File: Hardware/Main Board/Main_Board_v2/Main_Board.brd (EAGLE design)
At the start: 138.4 x 103.8 mm, 54 parts, among them IC1 MBED_MICROCONTROLLER, IC2 NE555, Q1 IRF3704, Q2 BS170

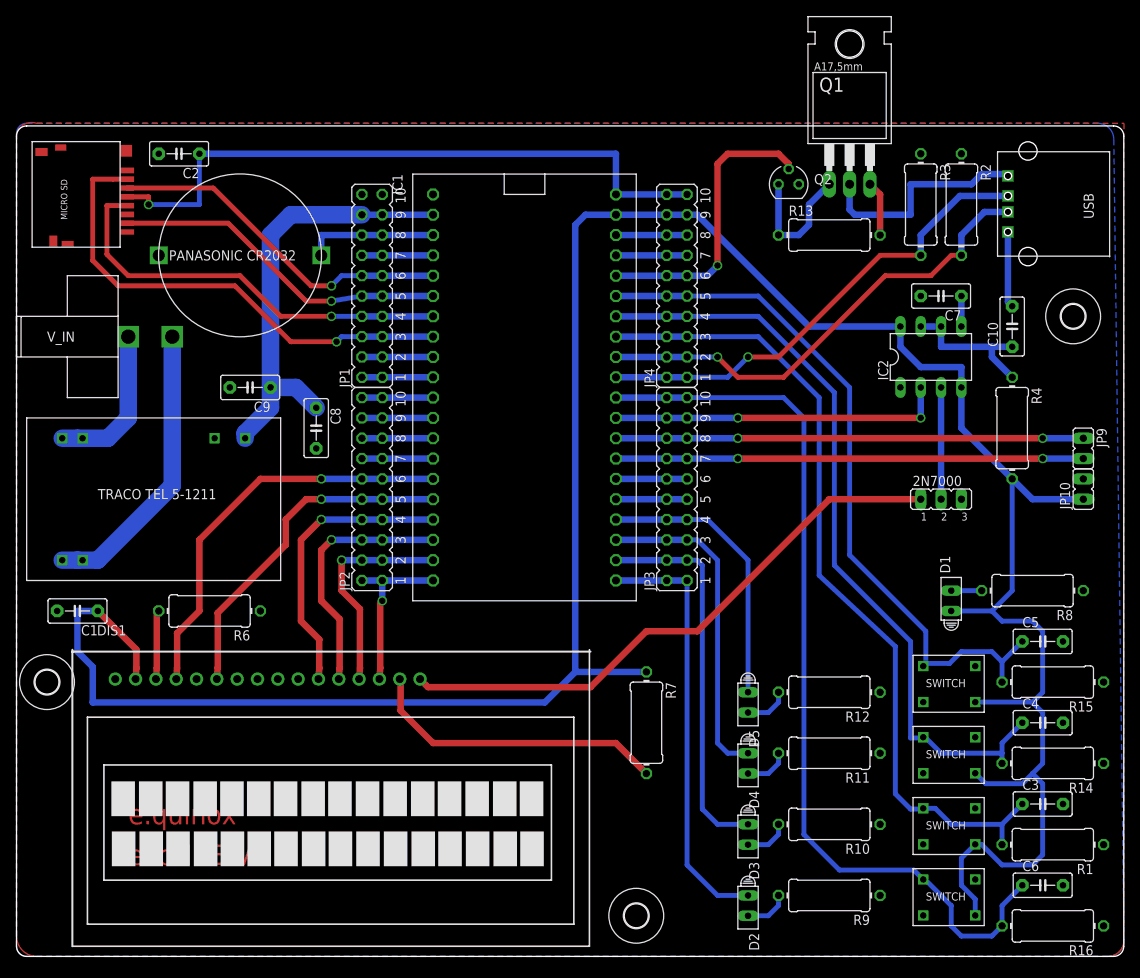
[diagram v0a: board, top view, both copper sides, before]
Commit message: Added Gerber Files for Main Board
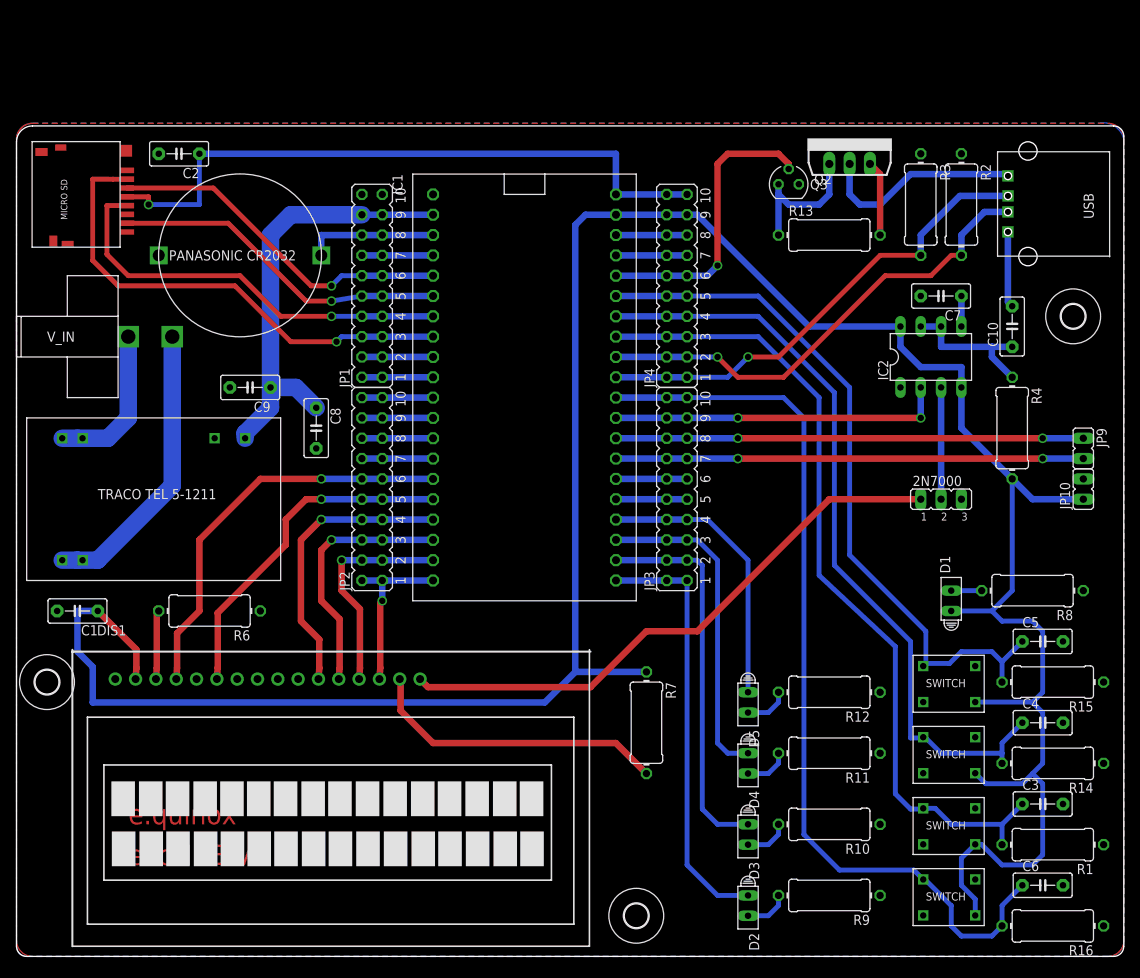
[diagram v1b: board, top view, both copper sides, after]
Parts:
- removed Q1: IRF3704, transistor-power:TO220AH
- added Q3: IRF3704L-V, transistor-power:TO262-V
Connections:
- net 5V: now also Q3.3; no longer Q1.E
- net MODEM: now also Q3.2; no longer Q1.C
- net N$5: now also Q3.1; no longer Q1.B
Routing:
- net 5V: track 6.88 -> 9.42 mm
- net MODEM: track 27.7 -> 25.8 mm
- net N$5: track 16.8 -> 17.6 mm
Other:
- outline, holes or cut-outs redrawn
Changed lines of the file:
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@@
 <board>
 <plain>
-<wire x1="1.27" y1="106.35" x2="1.27" y2="5.08" width="0" layer="20"/>
+<wire x1="138.41" y1="107.62" x2="3.27" y2="107.62" width="0" layer="20"/>
+<wire x1="3.27" y1="107.62" x2="1.27" y2="105.62" width="0" layer="20" curve="90"/>
+<wire x1="1.27" y1="105.62" x2="1.27" y2="5.08" width="0" layer="20"/>
 <wire x1="1.27" y1="5.08" x2="2.54" y2="3.81" width="0" layer="20" curve="90"/>
 <wire x1="2.54" y1="3.81" x2="138.41" y2="3.81" width="0" layer="20"/>
@@
 <wire x1="139.68" y1="5.08" x2="139.68" y2="106.35" width="0" layer="20"/>
 <wire x1="139.68" y1="106.35" x2="138.41" y2="107.62" width="0" layer="20" curve="90"/>
-<wire x1="138.41" y1="107.62" x2="2.54" y2="107.62" width="0" layer="20"/>
-<wire x1="2.54" y1="107.62" x2="1.27" y2="106.35" width="0" layer="20" curve="90"/>
 <dimension x1="139.68" y1="3.81" x2="139.68" y2="107.62" x3="149.86" y3="55.715" layer="20"/>
 <dimension x1="1.27" y1="3.81" x2="139.68" y2="3.81" x3="70.475" y3="-3.81" layer="20"/>
@@
 <element name="C2" library="capacitor-wima" package="C5B3" value="100nF" x="21.59" y="104.14" rot="R180"/>
 <element name="C3" library="capacitor-wima" package="C5B3" value="100nF" x="129.54" y="22.86"/>
-<element name="Q1" library="transistor-power" package="TO220AH" value="IRF3704" x="105.41" y="106.68"/>
 <element name="Q2" library="transistor-small-signal" package="SOT54E" value="BS170" x="97.79" y="100.33"/>
 <element name="R13" library="rcl" package="0411/12" value="1M" x="102.87" y="93.98"/>
@@
 <element name="U$11" library="holes" package="3,0" value="" x="133.35" y="83.82"/>
 <element name="U$12" library="holes" package="3,0" value="" x="5.08" y="38.1"/>
+<element name="Q3" library="transistor-power" package="TO262-V" value="IRF3704L-V" x="105.41" y="102.87"/>
 </elements>
 <signals>
@@
 <contactref element="C9" pad="2"/>
 <polygon width="0.4064" layer="1">
-<vertex x="1.27" y="6.35"/>
-<vertex x="1.27" y="106.68" curve="-90"/>
-<vertex x="3.81" y="107.95"/>
-<vertex x="139.7" y="107.95"/>
+<vertex x="137.7" y="3.81"/>
+<vertex x="3.27" y="3.81" curve="-90"/>
+<vertex x="1.27" y="5.81"/>
+<vertex x="1.27" y="105.95" curve="-90"/>
+<vertex x="3.27" y="107.95"/>
+<vertex x="137.7" y="107.95" curve="-90"/>
+<vertex x="139.7" y="105.95"/>
 <vertex x="139.7" y="5.81" curve="-90"/>
-<vertex x="137.7" y="3.81"/>
-<vertex x="3.81" y="3.81" curve="-90"/>
 </polygon>
 <polygon width="0.4064" layer="16">
-<vertex x="138.43" y="105.95"/>
+<vertex x="139.7" y="105.95"/>
 <vertex x="139.715984375" y="5.835609375" curve="-90.736003"/>
 <vertex x="137.716146875" y="3.810040625"/>
 <vertex x="2.54" y="3.81" curve="-90"/>
 <vertex x="1.27" y="5.08"/>
-<vertex x="1.27" y="106.68" curve="-90"/>
-<vertex x="2.54" y="107.95"/>
+<vertex x="1.27" y="105.95" curve="-90"/>
+<vertex x="3.27" y="107.95"/>
 <vertex x="136.43" y="107.95" curve="-90"/>
 </polygon>
@@
 </signal>
 <signal name="N$5">
-<contactref element="Q1" pad="B"/>
 <contactref element="Q2" pad="D"/>
 <contactref element="R13" pad="1"/>
-<wire x1="96.52" y1="93.98" x2="96.52" y2="100.33" width="0.8128" layer="16"/>
-<wire x1="100.33" y1="97.79" x2="102.87" y2="100.33" width="0.8128" layer="16"/>
-<wire x1="100.33" y1="97.79" x2="100.33" y2="95.25" width="0.8128" layer="16"/>
-<wire x1="100.33" y1="95.25" x2="99.06" y2="93.98" width="0.8128" layer="16"/>
-<wire x1="99.06" y1="93.98" x2="96.52" y2="93.98" width="0.8128" layer="16"/>
+<wire x1="96.52" y1="93.98" x2="96.52" y2="99.06" width="0.8128" layer="16"/>
+<contactref element="Q3" pad="1"/>
+<wire x1="96.52" y1="99.06" x2="96.52" y2="100.33" width="0.8128" layer="16"/>
+<wire x1="102.87" y1="102.87" x2="102.87" y2="99.06" width="0.8128" layer="16"/>
+<wire x1="102.87" y1="99.06" x2="101.6" y2="97.79" width="0.8128" layer="16"/>
+<wire x1="101.6" y1="97.79" x2="97.79" y2="97.79" width="0.8128" layer="16"/>
+<wire x1="97.79" y1="97.79" x2="96.52" y2="99.06" width="0.8128" layer="16"/>
 </signal>
 <signal name="5V">
-<contactref element="Q1" pad="E"/>
 <contactref element="R13" pad="2"/>
-<wire x1="109.22" y1="93.98" x2="109.22" y2="99.06" width="0.8128" layer="1"/>
-<wire x1="109.22" y1="99.06" x2="107.95" y2="100.33" width="0.8128" layer="1"/>
+<contactref element="Q3" pad="3"/>
+<wire x1="109.22" y1="93.98" x2="109.22" y2="101.6" width="0.8128" layer="1"/>
+<wire x1="109.22" y1="101.6" x2="107.95" y2="102.87" width="0.8128" layer="1"/>
 </signal>
 <signal name="MODEM">
-<contactref element="Q1" pad="C"/>
 <contactref element="U$1" pad="5V"/>
-<wire x1="105.41" y1="100.33" x2="105.41" y2="97.155" width="0.8128" layer="16"/>
-<wire x1="105.41" y1="97.155" x2="106.045" y2="96.52" width="0.8128" layer="16"/>
-<wire x1="106.045" y1="96.52" x2="113.03" y2="96.52" width="0.8128" layer="16"/>
-<wire x1="113.03" y1="96.52" x2="113.03" y2="100.33" width="0.8128" layer="16"/>
-<wire x1="113.03" y1="100.33" x2="120.65" y2="100.33" width="0.8128" layer="16"/>
-<wire x1="120.65" y1="100.33" x2="121.92" y2="101.6" width="0.8128" layer="16"/>
-<wire x1="121.92" y1="101.6" x2="124.97" y2="101.6" width="0.8128" layer="16"/>
+<wire x1="113.03" y1="101.6" x2="124.97" y2="101.6" width="0.8128" layer="16"/>
 <wire x1="124.97" y1="101.6" x2="125.2" y2="101.37" width="0.8128" layer="16"/>
+<contactref element="Q3" pad="2"/>
+<wire x1="113.03" y1="101.6" x2="109.22" y2="97.79" width="0.8128" layer="16"/>
+<wire x1="109.22" y1="97.79" x2="106.68" y2="97.79" width="0.8128" layer="16"/>
+<wire x1="106.68" y1="97.79" x2="105.41" y2="99.06" width="0.8128" layer="16"/>
+<wire x1="105.41" y1="99.06" x2="105.41" y2="102.87" width="0.8128" layer="16"/>
 </signal>
 <signal name="VIN-">
